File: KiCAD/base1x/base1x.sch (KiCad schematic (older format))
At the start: 39 parts, among them J1 Conn_02x05_Odd_Even, J2 GS3, J3 Conn_02x14_Counter_Clockwise, J4 GS3, J6 Conn_02x14_Counter_Clockwise, J7 Conn_02x06_Counter_Clockwise, J8 Conn_02x06_Counter_Clockwise, J9 Screw_Terminal_01x08, P3 CONN_01X02, P4 CONN_01X02, U1 ADS1115

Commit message: update kicad and add logos
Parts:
- J9: symbol Connector_Specialized:Screw_Terminal_01x08 -> Connector:Screw_Terminal_01x08
- L1: value GREY@CHRISTOFORO.NET -> grey@mutovis.com; footprint myParts:logo -> logo:logo_and_text; symbol myParts:GREY@CHRISTOFORO.NET -> logo:logo_text
- MK1, MK2: symbol Mechanical:Mounting_Hole_PAD -> Mechanical:MountingHole_Pad
- MK3, MK4, MK5, MK6, MK7, MK8: symbol Mechanical:Mounting_Hole -> Mechanical:MountingHole_Pad
- TP1, TP2, TP3, TP4, TP5, TP6: symbol Connector_Specialized:Test_Point -> Connector:TestPoint
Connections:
- no-connect marks 35 -> 41
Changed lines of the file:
@@
 V+
 $Comp
-L myParts:GREY@CHRISTOFORO.NET L1
+L logo:logo_text L1
 U 1 1 59B41702
-P 8950 7250
-F 0 "L1" H 8950 7125 60  0001 C CNN
-F 1 "GREY@CHRISTOFORO.NET" H 8950 7250 100 0000 C CNB
-F 2 "myParts:logo" H 8950 7250 60  0001 C CNN
-F 3 "" H 8950 7250 60  0001 C CNN
-	1    8950 7250
+P 9050 6800
+F 0 "L1" H 9050 6675 60  0001 C CNN
+F 1 "grey@mutovis.com" H 9000 6550 100 0000 C CNN
+F 2 "logo:logo_and_text" H 9050 6800 60  0001 C CNN
+F 3 "" H 9050 6800 60  0001 C CNN
+	1    9050 6800
 	1    0    0    -1
 $EndComp
@@
 External Power
 $Comp
-L Mechanical:Mounting_Hole_PAD MK1
+L Mechanical:MountingHole_Pad MK1
 U 1 1 59C916FE
 P 3300 6100
@@
 $EndComp
 $Comp
-L Mechanical:Mounting_Hole_PAD MK2
+L Mechanical:MountingHole_Pad MK2
 U 1 1 59C91760
 P 3300 6450
@@
 V_D_EXT
 $Comp
-L Connector_Specialized:Test_Point TP1
+L Connector:TestPoint TP1
 U 1 1 5A00C70E
 P 5650 6300
@@
 ~CS0
 $Comp
-L Connector_Specialized:Test_Point TP2
+L Connector:TestPoint TP2
 U 1 1 5A00C0AD
 P 4700 1850
@@
 I-R
 $Comp
-L Mechanical:Mounting_Hole MK3
+L Mechanical:MountingHole_Pad MK3
 U 1 1 5A00CBDC
 P 8800 1700
@@
 $EndComp
 $Comp
-L Mechanical:Mounting_Hole MK4
+L Mechanical:MountingHole_Pad MK4
 U 1 1 5A00CCA4
 P 8800 2050
@@
 $EndComp
 $Comp
-L Mechanical:Mounting_Hole MK5
+L Mechanical:MountingHole_Pad MK5
 U 1 1 5A00CCFE
 P 8800 2350
@@
 $EndComp
 $Comp
-L Mechanical:Mounting_Hole MK6
+L Mechanical:MountingHole_Pad MK6
 U 1 1 5A00CD58
 P 8800 2650
@@
 $EndComp
 $Comp
-L Mechanical:Mounting_Hole MK7
+L Mechanical:MountingHole_Pad MK7
 U 1 1 5A00CDAE
 P 8800 3000
@@
 $EndComp
 $Comp
-L Mechanical:Mounting_Hole MK8
+L Mechanical:MountingHole_Pad MK8
 U 1 1 5A00CE0E
 P 8800 3300
@@
 	4700 6750 4700 6450
 $Comp
-L Connector_Specialized:Screw_Terminal_01x08 J9
+L Connector:Screw_Terminal_01x08 J9
 U 1 1 5A36A6E7
 P 10150 1350
@@
 NoConn ~ 10050 1150
 $Comp
-L Connector_Specialized:Test_Point TP3
+L Connector:TestPoint TP3
 U 1 1 5A3700D5
 P 4250 2100
@@
 $EndComp
 $Comp
-L Connector_Specialized:Test_Point TP4
+L Connector:TestPoint TP4
 U 1 1 5A370173
 P 5000 2850
@@
 	5150 1200 4650 1200
 $Comp
-L Connector_Specialized:Test_Point TP5
+L Connector:TestPoint TP5
 U 1 1 5A371768
 P 5150 1200
@@
 This ADC will become ADS122C04 when it comes\nout to support analog inputs more negative than GND\nand I_sense will connect to AIN1
 $Comp
-L Connector_Specialized:Test_Point TP6
+L Connector:TestPoint TP6
 U 1 1 5A58BDB1
 P 10100 3850
@@
 Wire Wire Line
 	7250 2050 7500 2050
+NoConn ~ 8800 3400
+NoConn ~ 8800 3100
+NoConn ~ 8800 2750
+NoConn ~ 8800 2450
+NoConn ~ 8800 2150
+NoConn ~ 8800 1800
 $EndSCHEMATC

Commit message: MIT redesign in progress
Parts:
- removed J2, J4: GS3, Jumper:SolderJumper-3_P1.3mm_Open_RoundedPad1.0x1.5mm_NumberLabels, symbol Jumper:SolderJumper_3_Open
- removed JP2, JP3, JP4, JP5, JP6: Jumper_NO_Small, Jumper:SolderJumper-2_P1.3mm_Open_RoundedPad1.0x1.5mm, symbol Device:Jumper_NO_Small
- removed P3, P4: CONN_01X02, Connector_PinHeader_2.54mm:PinHeader_1x02_P2.54mm_Vertical, symbol Connector_Generic:Conn_01x02
- removed R5: 1, Resistor_SMD:R_2512_6332Metric, symbol Device:R
- removed U1: ADS1115, Package_SO:MSOP-10_3x3mm_P0.5mm, symbol myParts:ADS1115
- added C10, C9: 10uF, Capacitor_SMD:C_1206_3216Metric, symbol Device:C_Small
- added C11, C4, C7: 1000pF, Capacitor_SMD:C_1206_3216Metric, symbol Device:C_Small
- added C12, C13: 47uF, symbol Device:CP1_Small
- added C2, C3, C5, C6, C8: 0.1uF, Capacitor_SMD:C_1206_3216Metric, symbol Device:C_Small
- added J10, J11, J12, J13, J14, J16, J17, J2, J4, J5: Conn_01x03, symbol Connector_Generic:Conn_01x03
- added J15: Conn_01x08, symbol Connector_Generic:Conn_01x08
- added JP1, JP2: Jumper_NC_Small, Jumper:SolderJumper-2_P1.3mm_Open_RoundedPad1.0x1.5mm, symbol Device:Jumper_NC_Small
- added U2, U5: ads122c04, symbol myParts:ads122c04
- added U3, U6, U7: AD8615, Package_TO_SOT_SMD:TSOT-23-5, symbol Amplifier_Operational:AD8603
- added U4: NUP4202, Package_TO_SOT_SMD:SOT-363_SC-70-6, symbol Power_Protection:NUP4202
- added U8: LT1963AxQ-2.5, Package_TO_SOT_SMD:TO-263-5_TabPin3, symbol Regulator_Linear:LT1963AxQ-2.5
- added U9: LT3015xQ-2.5, Package_TO_SOT_SMD:TO-263-5_TabPin3, symbol Regulator_Linear:LT3015xQ-2.5
- C1: value 1uF -> 0.1uF
- D1, D2: C_D (none) -> 580pF; I_max (none) -> 20mA
- R1: value 1.2K -> 100R; farnellCode 2073370 -> 2073607
- R2: value 1.2K -> 100R; farnellCode 2073370 -> 2476379
- R3: value 10K -> 100R; farnellCode 2073607 -> 2476379
- R4: value 10K -> 2000R; farnellCode 2073607 -> 2476379
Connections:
- net labels added: +2V5, +5VA, -2V5, -5VA, GNDREF, V_Current, V_D1, V_D2
- net labels removed: I_sense, V_D_EXT, V_D_LOC
- wire segments 99 -> 247
- no-connect marks 41 -> 57
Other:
- note added: "Bias Voltage"
- note added: "Current Sense TIA"
- note added: "TRACO POWER TMR 6-0521"
- note removed: "Current Sense Resistor"
- note removed: "This ADC will become ADS122C04 when it comes\nout to support analog inputs more negative than GND\nand I_sense will connect to AIN1"
- moved on the sheet: D1, D2, J1, J7, J8, J9, MK1, MK2, MK3, MK4, MK5, MK6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

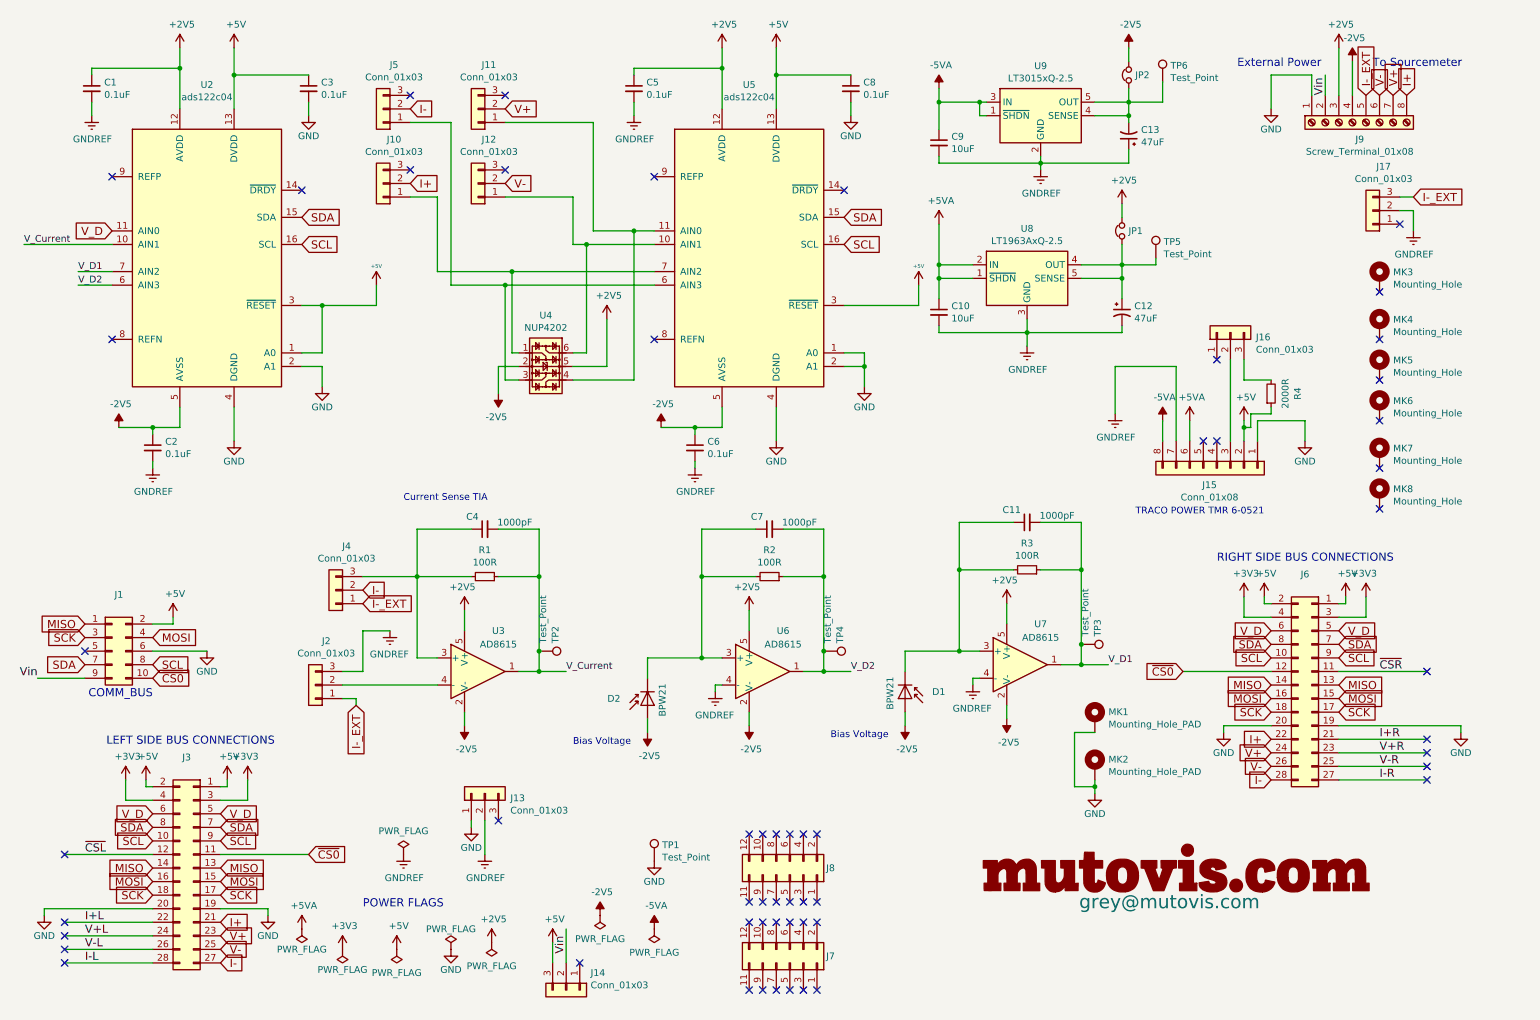
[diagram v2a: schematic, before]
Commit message: base 1x revisions
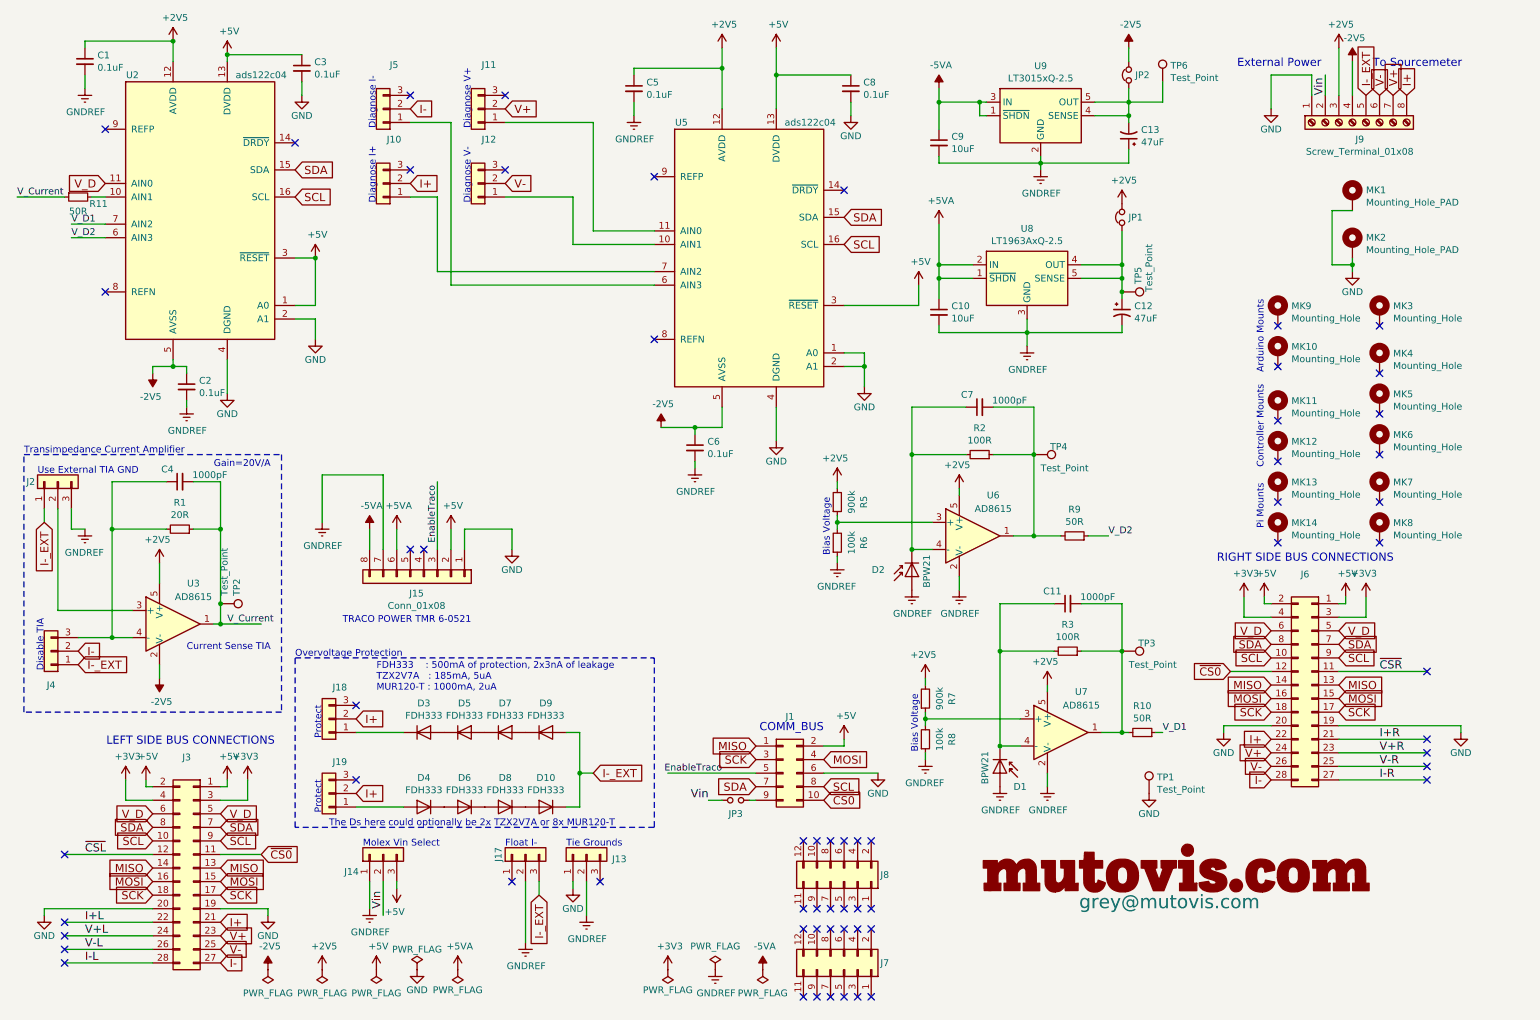
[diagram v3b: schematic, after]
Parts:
- removed J16: Conn_01x03, symbol Connector_Generic:Conn_01x03
- removed R4: 2000R, Resistor_SMD:R_1206_3216Metric, symbol Device:R_Small
- removed U4: NUP4202, Package_TO_SOT_SMD:SOT-363_SC-70-6, symbol Power_Protection:NUP4202
- added D10, D3, D4, D5, D6, D7, D8, D9: FDH333, Diode_THT:D_DO-35_SOD27_P7.62mm_Horizontal, symbol Diode:1N4148
- added J18, J19: Conn_01x03, symbol Connector_Generic:Conn_01x03
- added JP3: Jumper_NO_Small, symbol Device:Jumper_NO_Small
- added MK10, MK11, MK12, MK13, MK14, MK9: Mounting_Hole, MountingHole:MountingHole_3.2mm_M3, symbol Mechanical:MountingHole_Pad
- added R10, R11, R9: 50R, Resistor_SMD:R_1206_3216Metric, symbol Device:R_Small
- added R5, R7: 900k, Resistor_SMD:R_1206_3216Metric, symbol Device:R_Small
- added R6, R8: 100k, Resistor_SMD:R_1206_3216Metric, symbol Device:R_Small
- R1: value 100R -> 20R
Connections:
- net +2V5: now also R5.2, R7.2
- net -2V5: no longer D1.2 (A), D2.2 (A), U6.2 (V-), U7.2 (V-)
- net GNDREF: now also D1.2 (A), D2.2 (A), J14.1 (Pin_1), U6.2 (V-), U7.2 (V-), R6.1, R8.1; no longer U6.4 (-), U7.4 (-)
- net I+: now also J18.2 (Pin_2), J19.2 (Pin_2)
- net I-_EXT: now also D10.1 (K), D9.2 (A)
- net V_Current: now also R11.1; no longer U2.10 (AIN1)
- net V_D1: now also R10.1; no longer C11.2, R3.1, TP3.1, U7.1
- net V_D2: now also R9.1; no longer C7.2, R2.1, TP4.1, U6.1
- net Vin: now also JP3.1; no longer J1.9 (Pin_9)
- net EnableTraco: now reaches J1.5 (Pin_5)
- net EnableTraco: now also J15.3 (Pin_3)
- net at C11.1, D1.1 (K), R3.2: now also U7.4 (-); no longer U7.3 (+)
- net at C7.1, D2.1 (K), R2.2: now also U6.4 (-); no longer U6.3 (+)
- net at C4.1, J4.3 (Pin_3), R1.2: now also U3.4 (-); no longer U3.3 (+)
- net at J2.2 (Pin_2): now also U3.3 (+); no longer U3.4 (-)
- new net: J1.9 (Pin_9), JP3.2
- new net: C7.2, R2.1, R9.2, TP4.1, U6.1
- new net: R5.1, R6.2, U6.3 (+)
- new net: R7.1, R8.2, U7.3 (+)
- new net: C11.2, R10.2, R3.1, TP3.1, U7.1
- new net: R11.2, U2.10 (AIN1)
- new net: D3.1 (K), J18.1 (Pin_1)
- new net: D3.2 (A), D5.1 (K)
- new net: D5.2 (A), D7.1 (K)
- new net: D7.2 (A), D9.1 (K)
- new net: D10.2 (A), D8.1 (K)
- new net: D6.1 (K), D8.2 (A)
- new net: D4.1 (K), D6.2 (A)
- new net: D4.2 (A), J19.1 (Pin_1)
- no-connect marks 57 -> 62
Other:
- note added: "Arduino Mounts"
- note added: "Controller Mounts"
- note added: "Diagnose I+"
- note added: "Diagnose I-"
- note added: "Diagnose V+"
- note added: "Diagnose V-"
- note added: "Disable TIA"
- note added: "FDH333 : 500mA of protection, 2x3nA of leakage\nTZX2V7A : 185mA, 5uA\nMUR120-T : 1000mA, 2uA"
- note added: "Float I-"
- note added: "Gain=20V/A"
- note added: "Molex Vin Select"
- note added: "Overvoltage Protection"
- note added: "Pi Mounts"
- note added: "Protect"
- note added: "The Ds here could optionally be 2x TZX2V7A or 8x MUR120-T"
- note added: "Tie Grounds"
- note added: "Transimpedance Current Amplifier"
- note added: "Use External TIA GND"
- note removed: "POWER FLAGS"
- moved on the sheet: C1, C11, C2, C3, C4, C7, D1, D2, J1, J13, J14, J15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
